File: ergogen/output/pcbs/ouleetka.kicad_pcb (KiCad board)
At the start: 2 copper layers, 144.6 x 93.8 mm, 66 parts

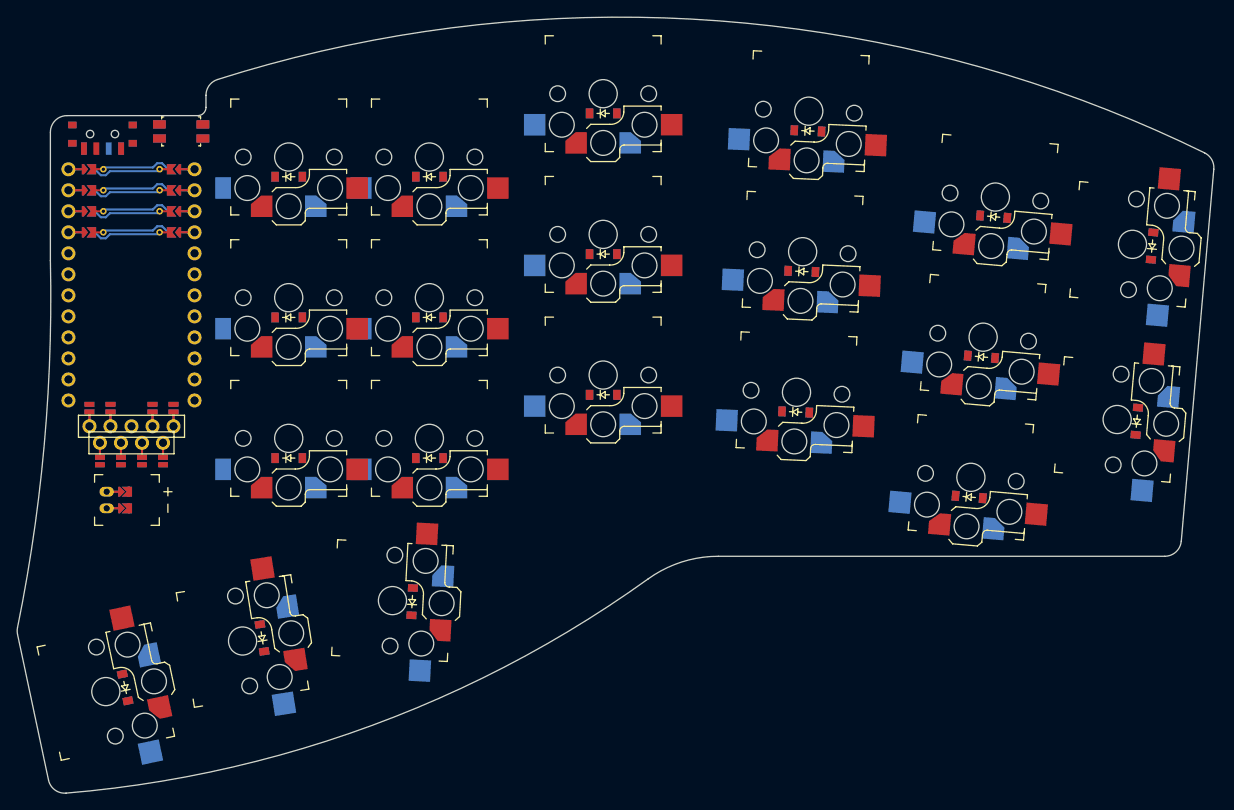
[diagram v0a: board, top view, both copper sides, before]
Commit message: refactoring
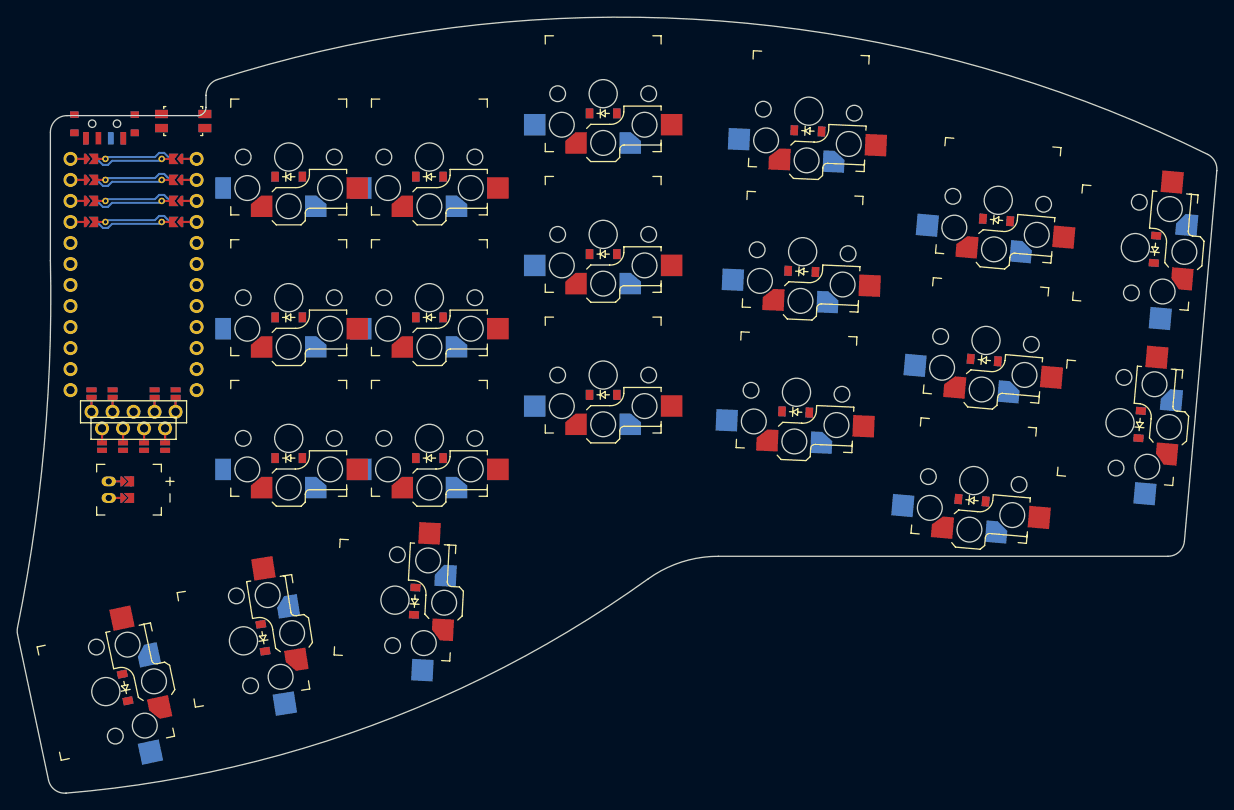
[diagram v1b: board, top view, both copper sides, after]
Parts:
- moved DISP1 1.77 mm to (81.2, 80.1)
- moved DISP2 1.77 mm to (81.2, 82.1)
- moved JST1 1.27 mm to (78.2, 106.2)
- moved MCU1 1.27 mm to (81.2, 78.9)
- moved PWR1 1.27 mm to (77.8, 62.0)
- moved RST1 1.27 mm to (87.2, 61.7)
- moved D13 0.52 mm to (182.6, 107.5)
- moved D16 0.52 mm to (202.8, 98.3)
- moved D17 0.52 mm to (204.7, 77.2)
- moved D33 0.52 mm to (182.6, 107.5)
- moved D36 0.52 mm to (202.8, 98.3)
- moved D37 0.52 mm to (204.7, 77.2)
- moved S10 0.52 mm to (182.8, 105.1)
- moved S16 0.52 mm to (200.5, 98.1)
- moved S17 0.52 mm to (202.3, 76.9)
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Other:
- board size 144.6 x 93.8 mm -> 145 x 93.8 mm

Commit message: outlines refactoring
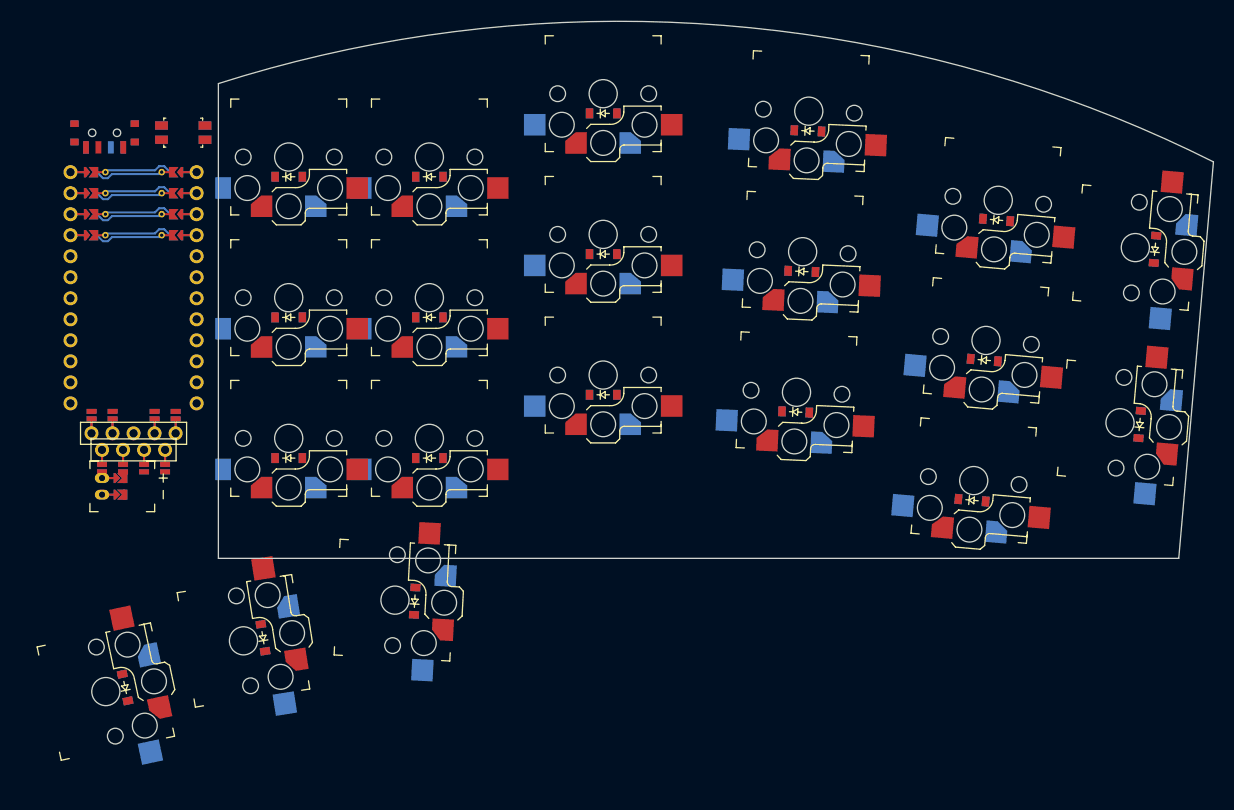
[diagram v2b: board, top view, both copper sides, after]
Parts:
- moved DISP1 2.60 mm to (81.2, 82.7)
- moved DISP2 2.60 mm to (81.2, 84.7)
- moved MCU1 1.60 mm to (81.2, 80.5)
- moved RST1 1.40 mm to (87.2, 63.1)
- moved PWR1 1.10 mm to (77.8, 63.1)
- moved JST1 0.90 mm to (77.4, 105.8)
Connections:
- net inner_thome renamed inner_default
- net middle_thome renamed middle_default
- net outer_thome renamed outer_default
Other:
- board size 145 x 93.8 mm -> 120.2 x 64.9 mm
